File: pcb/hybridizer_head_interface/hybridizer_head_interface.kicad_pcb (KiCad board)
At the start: 2 copper layers, 85.6 x 132.2 mm, 126 parts, among them P1 HEADER_02X07_SMD, P2 HEADER_02X05_SMD, P3 HEADER_02X05_SMD, U1 VA, U11 VA, U13 VA, U15 DRV103, U16 DRV103, U17 DRV103, U18 DRV103, U19 DRV103, U20 DRV103, U21 DRV103, U22 DRV103, U23 OA, U24 OA, U25 OA, U26 OA, U27 OA, U28 OA, U29 OA, U3 VA, U5 VA, U7 VA, U9 VA

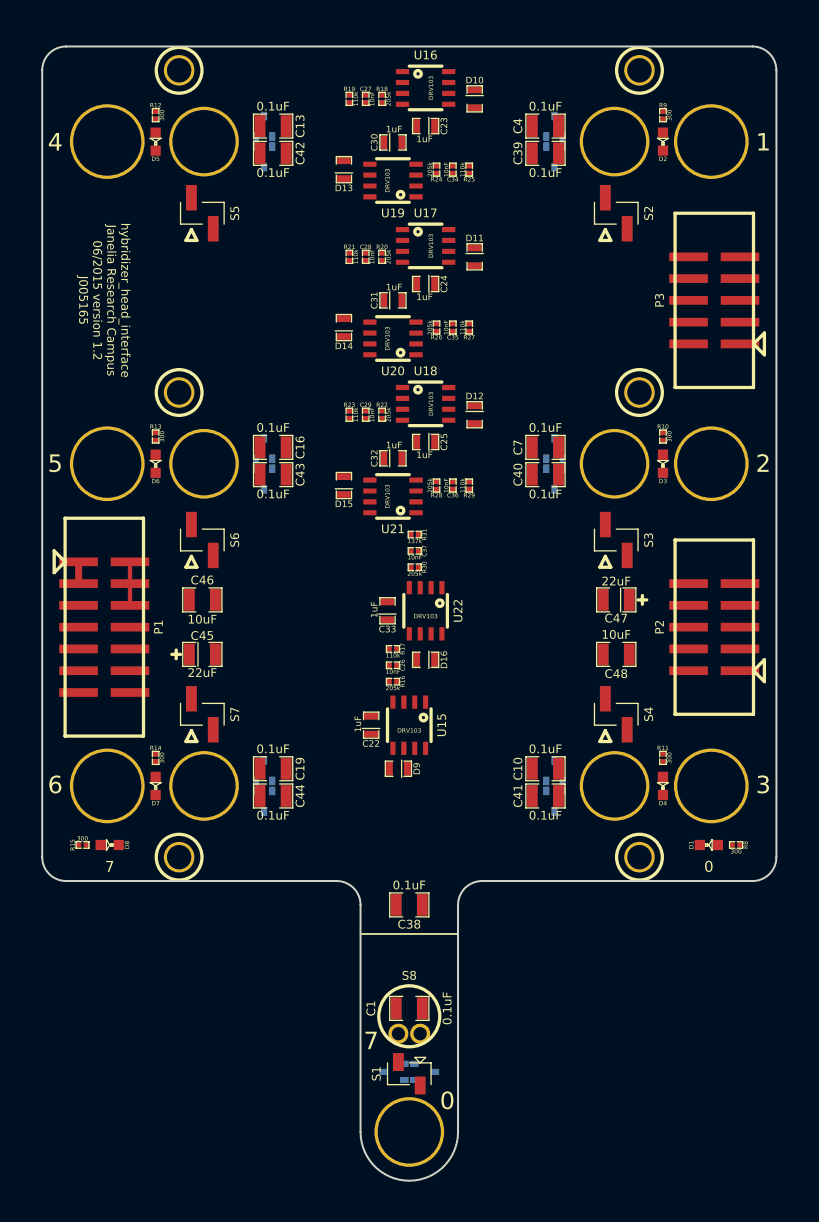
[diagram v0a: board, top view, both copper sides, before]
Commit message: Finished hybridizer_head_interface_v1.2.
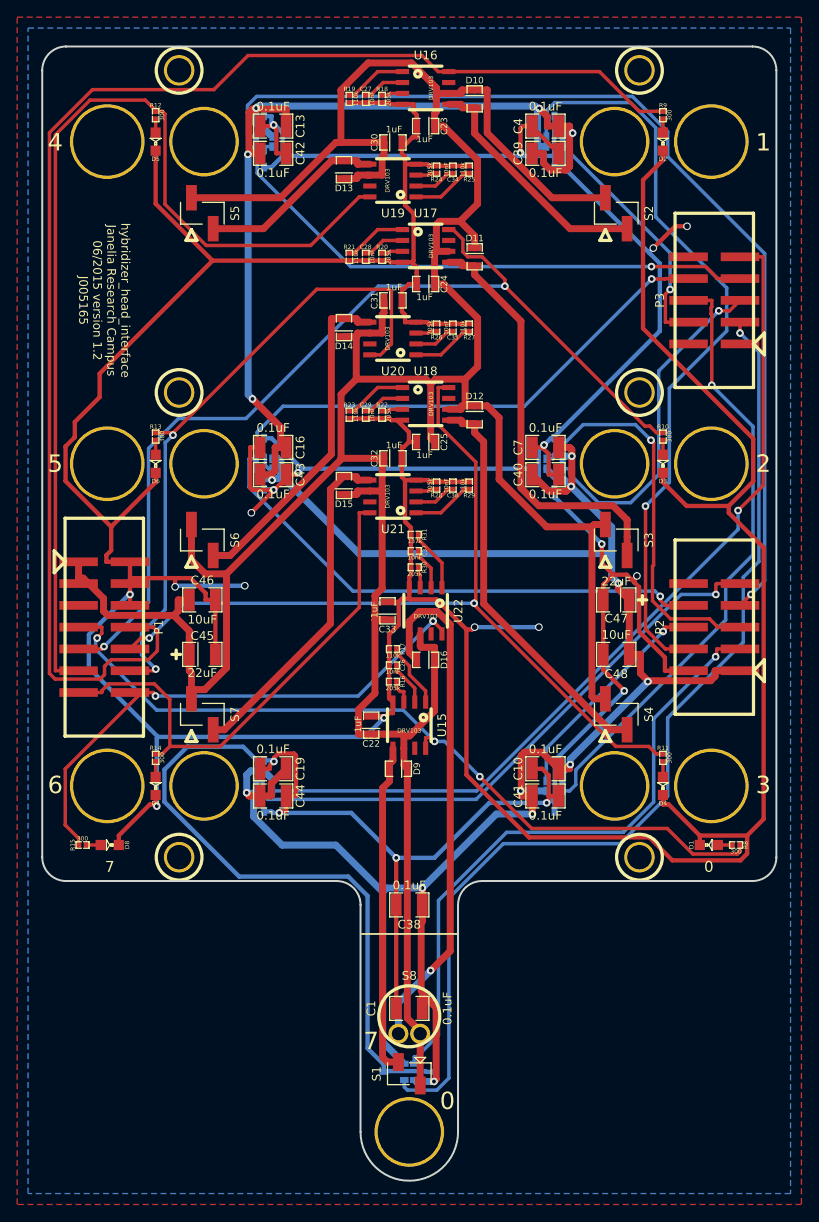
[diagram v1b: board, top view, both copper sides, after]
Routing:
- net GND: track 5.08 -> 487.3 mm, vias 0 -> 7
- net VAA: track 2.54 -> 408.7 mm
- net GNDA: track 0.00 -> 390.6 mm, vias 0 -> 15
- net +5V: track 0.00 -> 360.5 mm, vias 0 -> 16
- net /IO1: track 0.00 -> 161.5 mm
- net /IO4: track 0.00 -> 119.2 mm
- net /A8: track 0.00 -> 118.7 mm, vias 0 -> 1
- net /A4: track 0.00 -> 116.7 mm, vias 0 -> 1
- net /IO2: track 0.00 -> 113.8 mm, vias 0 -> 2
- net /A14: track 0.00 -> 102.6 mm, vias 0 -> 1
- net /IO3: track 0.00 -> 100.0 mm, vias 0 -> 2
- net /IO0: track 0.00 -> 93.9 mm, vias 0 -> 3
- net /A1: track 0.00 -> 89.2 mm, vias 0 -> 1
- net /IO5: track 0.00 -> 76.5 mm, vias 0 -> 2
- net /A0: track 0.00 -> 73.8 mm, vias 0 -> 1
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- added copper zone on F.Cu, net GND
- added copper zone on B.Cu, net GNDA
